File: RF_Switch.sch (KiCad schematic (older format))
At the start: 5 parts, among them J1 Conn_Coaxial, J2 Conn_01x04, J3 Conn_Coaxial, J4 Conn_Coaxial, U1 HSWA2-30DR+

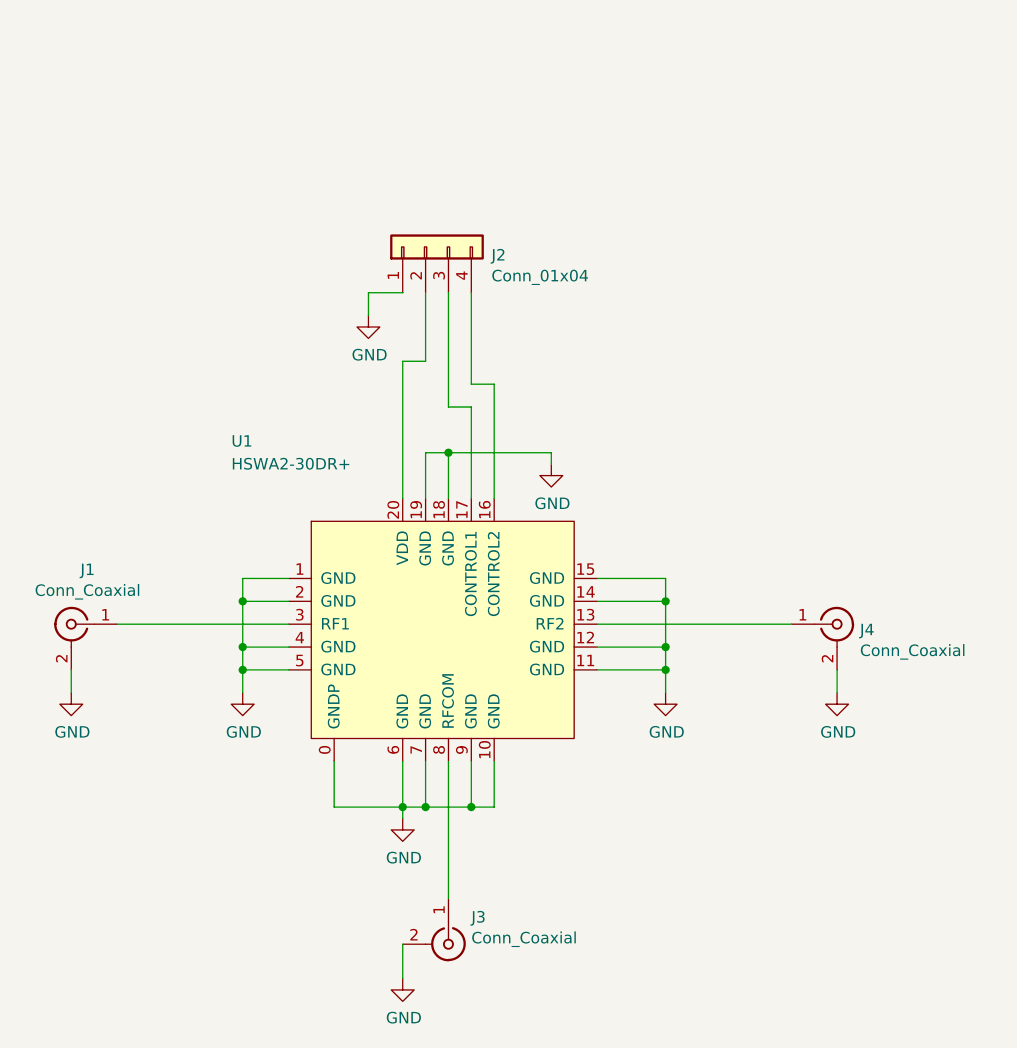
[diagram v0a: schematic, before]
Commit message: Finished REV A
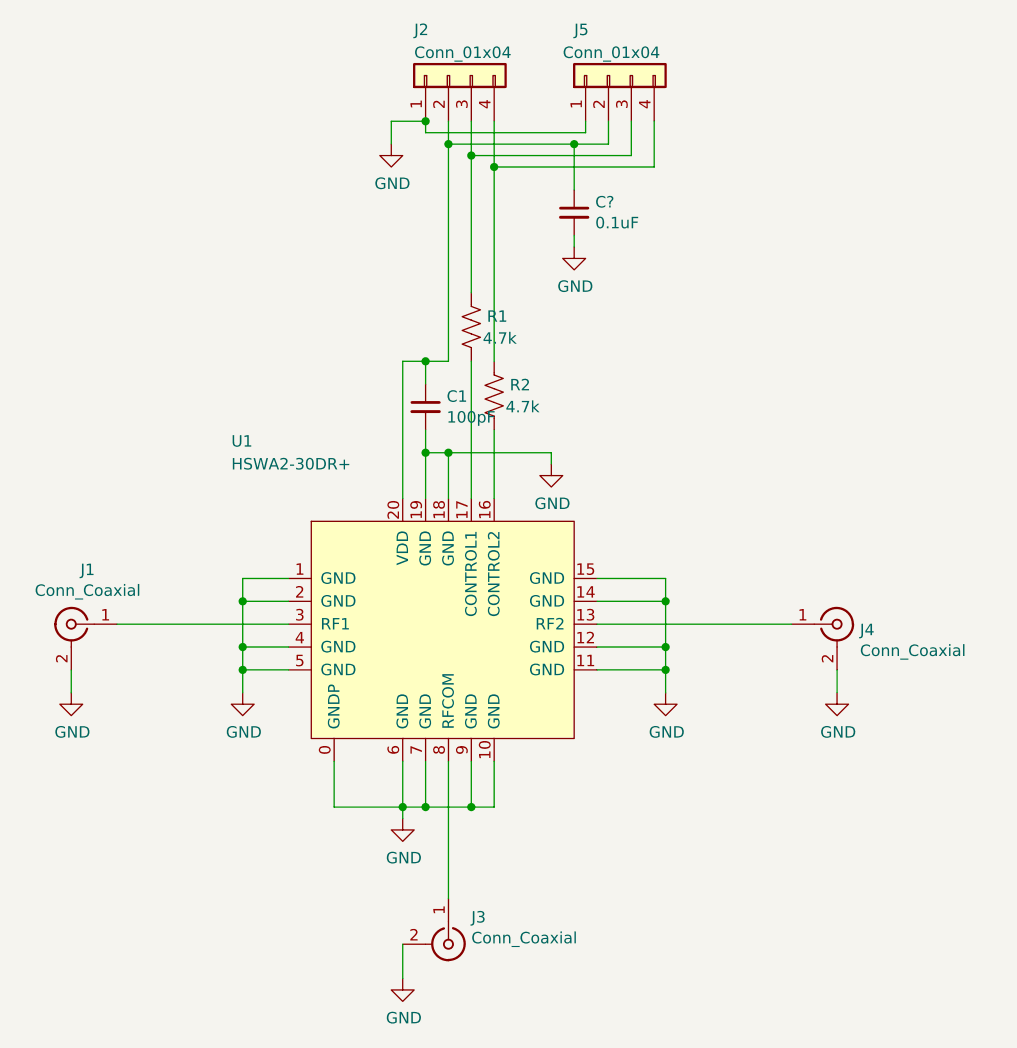
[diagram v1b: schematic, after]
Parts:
- added C1: 100pF, Capacitor_SMD:C_0603_1608Metric, symbol LSR_SCH_LIB:C_Small
- added C?: 0.1uF, Capacitor_SMD:C_0603_1608Metric, symbol LSR_SCH_LIB:C_Small
- added J5: Conn_01x04, lib_fp:Header 4 Keyed RT Angle, symbol Connector_Generic:Conn_01x04
- added R1, R2: 4.7k, Resistor_SMD:R_0603_1608Metric, symbol Device:R_US
- J1, J4: footprint Connector_Coaxial:SMA_Amphenol_132289_EdgeMount -> lib_fp:SMA_Taoglas_Limited_Narrow_EdgeMount; Digikey Part Number (none) -> 931-1175-ND
- J3: footprint Connector_Coaxial:SMA_Amphenol_132289_EdgeMount -> lib_fp:SMA_Plug_Linx_Technologies_EdgeMount_CONSMA013.062; Digikey Part Number (none) -> CONSMA013.062-ND
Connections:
- net GND: now also C1.2, C?.2, J5.1 (Pin_1)
- net at U1.16 (CONTROL2): now also R2.2; no longer J2.4 (Pin_4)
- net at U1.17 (CONTROL1): now also R1.2; no longer J2.3 (Pin_3)
- net at J2.2 (Pin_2), U1.20 (VDD): now also C1.1, C?.1, J5.2 (Pin_2)
- new net: J2.3 (Pin_3), J5.3 (Pin_3), R1.1
- new net: J2.4 (Pin_4), J5.4 (Pin_4), R2.1
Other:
- moved on the sheet: J2
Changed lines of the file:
@@
 F 0 "J4" H 7850 3725 50  0000 L CNN
 F 1 "Conn_Coaxial" H 7850 3634 50  0000 L CNN
-F 2 "Connector_Coaxial:SMA_Amphenol_132289_EdgeMount" H 7750 3750 50  0001 C CNN
+F 2 "lib_fp:SMA_Taoglas_Limited_Narrow_EdgeMount" H 7750 3750 50  0001 C CNN
 F 3 " ~" H 7750 3750 50  0001 C CNN
+F 4 "931-1175-ND" H 7750 3750 50  0001 C CNN "Digikey Part Number"
 	1    7750 3750
 	1    0    0    -1
@@
 F 0 "J3" V 5932 5250 50  0000 L CNN
 F 1 "Conn_Coaxial" V 6023 5250 50  0000 L CNN
-F 2 "Connector_Coaxial:SMA_Amphenol_132289_EdgeMount" H 6050 5150 50  0001 C CNN
+F 2 "lib_fp:SMA_Plug_Linx_Technologies_EdgeMount_CONSMA013.062" H 6050 5150 50  0001 C CNN
 F 3 " ~" H 6050 5150 50  0001 C CNN
+F 4 "CONSMA013.062-ND" V 6050 5150 50  0001 C CNN "Digikey Part Number"
 	1    6050 5150
 	0    1    1    0
@@
 F 0 "J1" H 4328 3988 50  0000 C CNN
 F 1 "Conn_Coaxial" H 4328 3897 50  0000 C CNN
-F 2 "Connector_Coaxial:SMA_Amphenol_132289_EdgeMount" H 4400 3750 50  0001 C CNN
+F 2 "lib_fp:SMA_Taoglas_Limited_Narrow_EdgeMount" H 4400 3750 50  0001 C CNN
 F 3 " ~" H 4400 3750 50  0001 C CNN
+F 4 "931-1175-ND" H 4400 3750 50  0001 C CNN "Digikey Part Number"
 	1    4400 3750
 	-1   0    0    -1
@@
 	7000 3850 7000 3650
 Wire Wire Line
-	5950 3200 5950 3000
-Wire Wire Line
 	5950 3000 6050 3000
 Wire Wire Line
 	6050 3000 6050 3200
 Wire Wire Line
-	5850 3200 5850 2600
-Wire Wire Line
-	5850 2600 5950 2600
-Wire Wire Line
-	5950 2600 5950 2300
-Wire Wire Line
-	6150 3200 6150 2800
-Wire Wire Line
-	6150 2800 6050 2800
-Wire Wire Line
-	6050 2800 6050 2300
-Wire Wire Line
-	6150 2300 6150 2700
-Wire Wire Line
-	6150 2700 6250 2700
-Wire Wire Line
-	6250 2700 6250 3200
+	6250 1550 6250 1750
 Wire Wire Line
 	5850 4600 5850 4550
@@
 L Connector_Generic:Conn_01x04 J2
 U 1 1 5EBA926A
-P 5950 2100
-F 0 "J2" V 5914 1812 50  0000 R CNN
-F 1 "Conn_01x04" V 5823 1812 50  0000 R CNN
-F 2 "lib_fp:Header 4 Keyed RT Angle" H 5950 2100 50  0001 C CNN
-F 3 "~" H 5950 2100 50  0001 C CNN
-	1    5950 2100
+P 6050 1350
+F 0 "J2" V 6250 1500 50  0000 R CNN
+F 1 "Conn_01x04" V 6150 1500 50  0000 R CNN
+F 2 "lib_fp:Header 4 Keyed RT Angle" H 6050 1350 50  0001 C CNN
+F 3 "~" H 6050 1350 50  0001 C CNN
+	1    6050 1350
 	0    -1   -1   0
 $EndComp
@@
 L power:GND #PWR0108
 U 1 1 5EBAA03E
-P 5700 2400
-F 0 "#PWR0108" H 5700 2150 50  0001 C CNN
-F 1 "GND" H 5705 2227 50  0000 C CNN
-F 2 "" H 5700 2400 50  0001 C CNN
-F 3 "" H 5700 2400 50  0001 C CNN
-	1    5700 2400
-	1    0    0    -1
-$EndComp
-Wire Wire Line
-	5700 2400 5700 2300
-Wire Wire Line
-	5700 2300 5850 2300
+P 5800 1650
+F 0 "#PWR0108" H 5800 1400 50  0001 C CNN
+F 1 "GND" H 5805 1477 50  0000 C CNN
+F 2 "" H 5800 1650 50  0001 C CNN
+F 3 "" H 5800 1650 50  0001 C CNN
+	1    5800 1650
+	1    0    0    -1
+$EndComp
+Wire Wire Line
+	5800 1650 5800 1550
+Wire Wire Line
+	5800 1550 5950 1550
 Wire Wire Line
 	5550 4350 5550 4550
 Wire Wire Line
 	5550 4550 5850 4550
+$Comp
+L Connector_Generic:Conn_01x04 J5
+U 1 1 5EBC0BC2
+P 6750 1350
+F 0 "J5" V 6950 1500 50  0000 R CNN
+F 1 "Conn_01x04" V 6850 1550 50  0000 R CNN
+F 2 "lib_fp:Header 4 Keyed RT Angle" H 6750 1350 50  0001 C CNN
+F 3 "~" H 6750 1350 50  0001 C CNN
+	1    6750 1350
+	0    -1   -1   0
+$EndComp
+Wire Wire Line
+	6650 1550 6650 1600
+Wire Wire Line
+	6650 1600 5950 1600
+Wire Wire Line
+	5950 1600 5950 1550
+Connection ~ 5950 1550
+Wire Wire Line
+	6750 1550 6750 1650
+Wire Wire Line
+	6750 1650 6600 1650
+Connection ~ 6050 1650
+Wire Wire Line
+	6050 1650 6050 1550
+Wire Wire Line
+	6850 1550 6850 1700
+Wire Wire Line
+	6850 1700 6150 1700
+Wire Wire Line
+	6150 1700 6150 1550
+Wire Wire Line
+	6950 1550 6950 1750
+Wire Wire Line
+	6950 1750 6250 1750
+$Comp
+L Device:R_US R2
+U 1 1 5EBC8643
+P 6250 2750
+F 0 "R2" H 6318 2796 50  0000 L CNN
+F 1 "4.7k" H 6300 2700 50  0000 L CNN
+F 2 "Resistor_SMD:R_0603_1608Metric" V 6290 2740 50  0001 C CNN
+F 3 "~" H 6250 2750 50  0001 C CNN
+	1    6250 2750
+	1    0    0    -1
+$EndComp
+$Comp
+L Device:R_US R1
+U 1 1 5EBCD126
+P 6150 2450
+F 0 "R1" H 6218 2496 50  0000 L CNN
+F 1 "4.7k" H 6200 2400 50  0000 L CNN
+F 2 "Resistor_SMD:R_0603_1608Metric" V 6190 2440 50  0001 C CNN
+F 3 "~" H 6150 2450 50  0001 C CNN
+	1    6150 2450
+	1    0    0    -1
+$EndComp
+Wire Wire Line
+	6250 3200 6250 2900
+Wire Wire Line
+	6150 2600 6150 3200
+Wire Wire Line
+	6050 2600 5950 2600
+Wire Wire Line
+	5850 2600 5850 3200
+Wire Wire Line
+	6050 1650 6050 2600
+$Comp
+L LSR_SCH_LIB:C_Small C1
+U 1 1 5EBD55E6
+P 5950 2800
+F 0 "C1" H 6042 2846 50  0000 L CNN
+F 1 "100pF" H 6042 2755 50  0000 L CNN
+F 2 "Capacitor_SMD:C_0603_1608Metric" H 5950 2800 50  0001 C CNN
+F 3 "~" H 5950 2800 50  0001 C CNN
+	1    5950 2800
+	1    0    0    -1
+$EndComp
+Wire Wire Line
+	5950 2700 5950 2600
+Connection ~ 5950 2600
+Wire Wire Line
+	5950 2600 5850 2600
+Wire Wire Line
+	5950 2900 5950 3000
+Connection ~ 5950 3000
+Wire Wire Line
+	5950 3000 5950 3200
+Connection ~ 6250 1750
+Wire Wire Line
+	6250 1750 6250 2600
+Connection ~ 6150 1700
+Wire Wire Line
+	6150 1700 6150 2300
+$Comp
+L LSR_SCH_LIB:C_Small C?
+U 1 1 5EBE0161
+P 6600 1950
+F 0 "C?" H 6692 1996 50  0000 L CNN
+F 1 "0.1uF" H 6692 1905 50  0000 L CNN
+F 2 "Capacitor_SMD:C_0603_1608Metric" H 6600 1950 50  0001 C CNN
+F 3 "~" H 6600 1950 50  0001 C CNN
+	1    6600 1950
+	1    0    0    -1
+$EndComp
+$Comp
+L power:GND #PWR?
+U 1 1 5EBE0E04
+P 6600 2100
+F 0 "#PWR?" H 6600 1850 50  0001 C CNN
+F 1 "GND" H 6605 1927 50  0000 C CNN
+F 2 "" H 6600 2100 50  0001 C CNN
+F 3 "" H 6600 2100 50  0001 C CNN
+	1    6600 2100
+	1    0    0    -1
+$EndComp
+Wire Wire Line
+	6600 2100 6600 2050
+Wire Wire Line
+	6600 1850 6600 1650
+Connection ~ 6600 1650
+Wire Wire Line
+	6600 1650 6050 1650
 $EndSCHEMATC
